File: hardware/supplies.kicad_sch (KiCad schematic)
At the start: 29 parts, among them J11 Conn_01x02, J12 Conn_01x02, U5 AMS1117-3.3, U8 LM5017MR

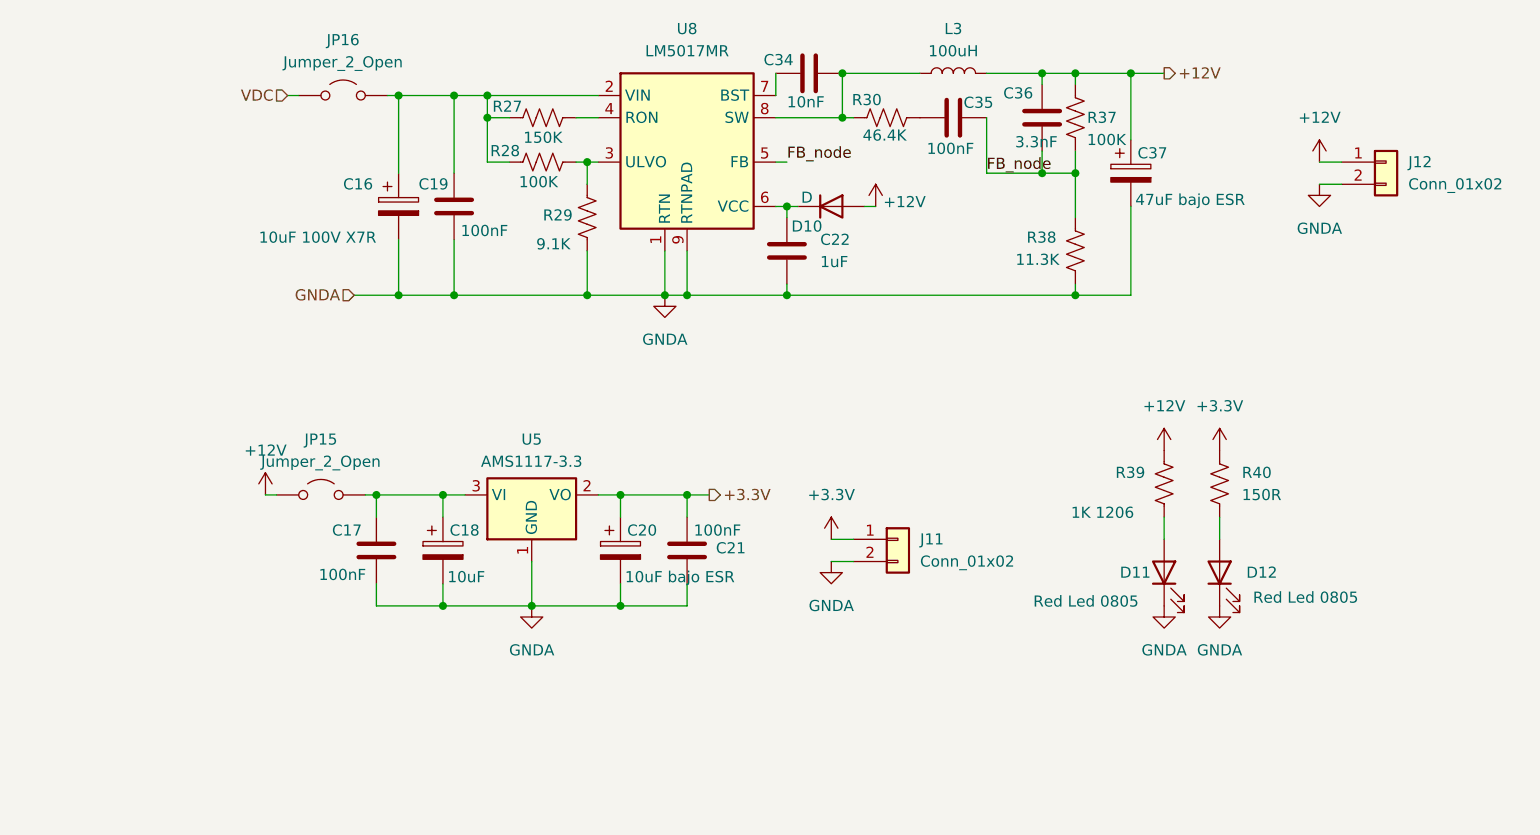
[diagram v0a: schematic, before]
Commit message: HW: Sch done. PCB WIP
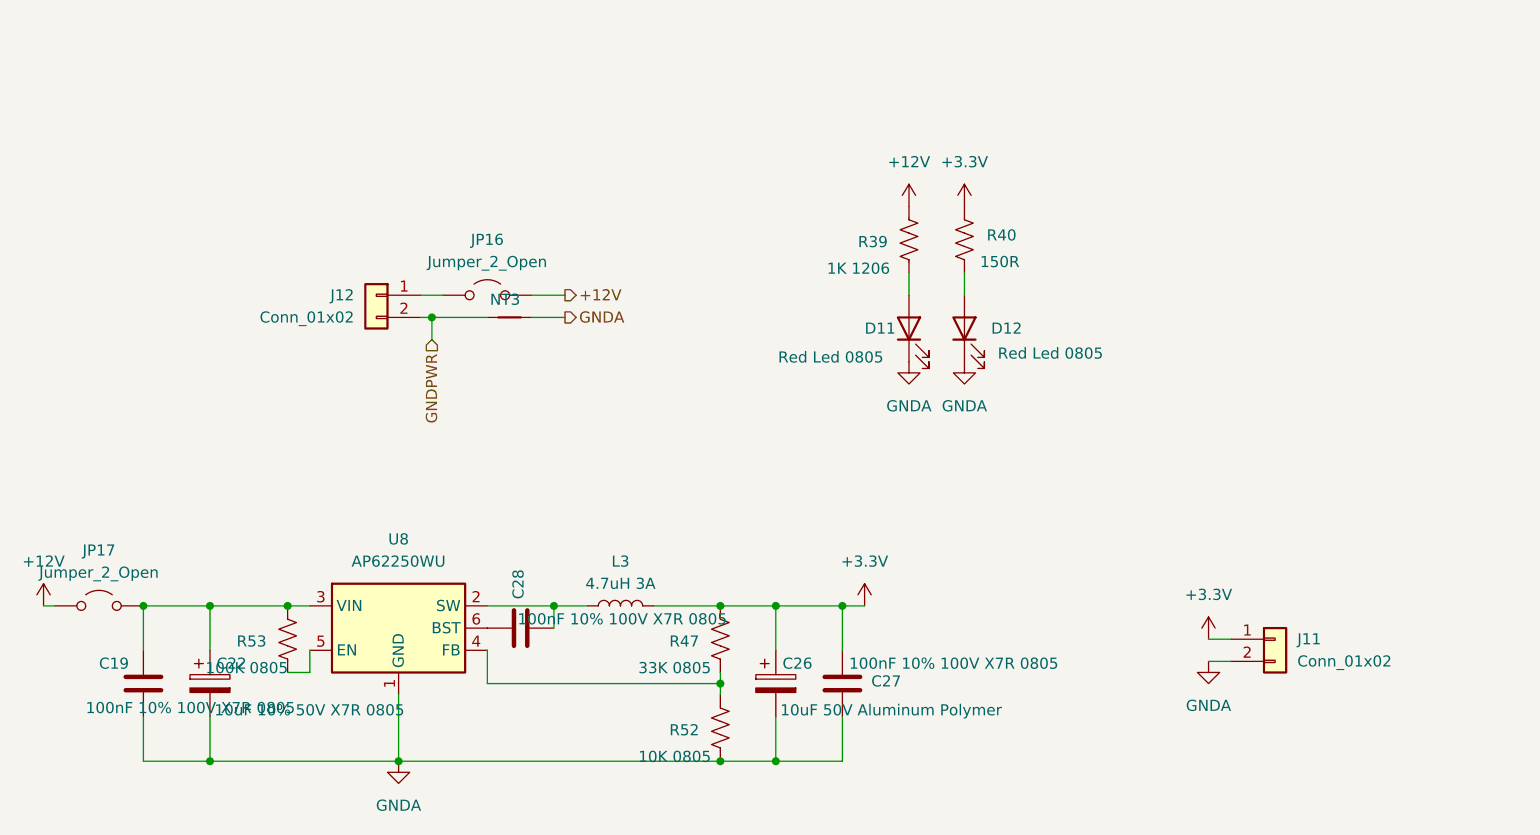
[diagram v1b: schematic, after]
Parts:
- removed C16: 10uF 100V X7R, symbol Device:C_Polarized
- removed C17, C21, C35: 100nF, symbol Device:C
- removed C18: 10uF, symbol Device:C_Polarized
- removed C20: 10uF bajo ESR, symbol Device:C_Polarized
- removed C22: 1uF, symbol Device:C
- removed C34: 10nF, symbol Device:C
- removed C36: 3.3nF, symbol Device:C
- removed C37: 47uF bajo ESR, symbol Device:C_Polarized
- removed D10: D, symbol Device:D
- removed JP15: Jumper_2_Open, symbol Jumper:Jumper_2_Open
- removed R27: 150K, symbol Device:R_US
- removed R28, R37: 100K, symbol Device:R_US
- removed R29: 9.1K, symbol Device:R_US
- removed R30: 46.4K, symbol Device:R_US
- removed R38: 11.3K, symbol Device:R_US
- removed U5: AMS1117-3.3, Package_TO_SOT_SMD:SOT-223-3_TabPin2, symbol Regulator_Linear:AMS1117-3.3
- removed U8: LM5017MR, Package_SO:SOIC-8-1EP_3.9x4.9mm_P1.27mm_EP2.95x4.9mm_Mask2.71x3.4mm_ThermalVias, symbol Regulator_Switching:LM5017MR
- added C22: 10uF 10% 50V X7R 0805, Capacitor_SMD:C_0805_2012Metric_Pad1.18x1.45mm_HandSolder, symbol Device:C_Polarized
- added C26: 10uF 50V Aluminum Polymer, Capacitor_THT:CP_Radial_D6.3mm_P2.50mm, symbol Device:C_Polarized
- added C27, C28: 100nF 10% 100V X7R 0805, Capacitor_SMD:C_0805_2012Metric_Pad1.18x1.45mm_HandSolder, symbol Device:C
- added JP17: Jumper_2_Open, Connector_PinHeader_2.54mm:PinHeader_1x02_P2.54mm_Vertical, symbol Jumper:Jumper_2_Open
- added NT3: NetTie_2, NetTie:NetTie-2_SMD_Pad2.0mm, symbol Device:NetTie_2
- added R47: 33K 0805, Resistor_SMD:R_0805_2012Metric_Pad1.20x1.40mm_HandSolder, symbol Device:R_US
- added R52: 10K 0805, Resistor_SMD:R_0805_2012Metric_Pad1.20x1.40mm_HandSolder, symbol Device:R_US
- added R53: 100K 0805, Resistor_SMD:R_0805_2012Metric_Pad1.20x1.40mm_HandSolder, symbol Device:R_US
- added U8: AP62250WU, Package_TO_SOT_SMD:TSOT-23-6, symbol Regulator_Switching:AP62250WU
- C19: value 100nF -> 100nF 10% 100V X7R 0805; footprint (none) -> Capacitor_SMD:C_0805_2012Metric_Pad1.18x1.45mm_HandSolder
- J11, J12, JP16: footprint (none) -> Connector_PinHeader_2.54mm:PinHeader_1x02_P2.54mm_Vertical; now left out of the parts list
- L3: value 100uH -> 4.7uH 3A
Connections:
- net VDC is gone; now on net +12V: JP16.1 (A)
- net +12V: now also JP17.1 (A); no longer J12.1 (Pin_1), L3.2
- net +3.3V: now also L3.2, C26.1, C27.1, R47.1
- net GNDA: now also C22.2, C26.2, C27.2, NT3.2, R52.2, U8.1 (GND); no longer J12.2 (Pin_2)
- net at JP16.2 (B): now also J12.1 (Pin_1); no longer C19.1
- net at L3.1: now also C28.2, U8.2 (SW)
- new net: R47.2, R52.1, U8.4 (FB)
- new net: C28.1, U8.6 (BST)
- new net: C19.1, C22.1, JP17.2 (B), R53.1, U8.3 (VIN)
- new net: R53.2, U8.5 (EN)
- new net GNDPWR: J12.2 (Pin_2), NT3.1
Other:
- moved on the sheet: D11, D12, J11, J12, R39, R40
